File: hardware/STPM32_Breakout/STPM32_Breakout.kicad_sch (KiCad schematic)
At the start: 32 parts, among them J1 BREADBOARD I/O, SW1 RESET, U1 STPM32, Y1 16MHz

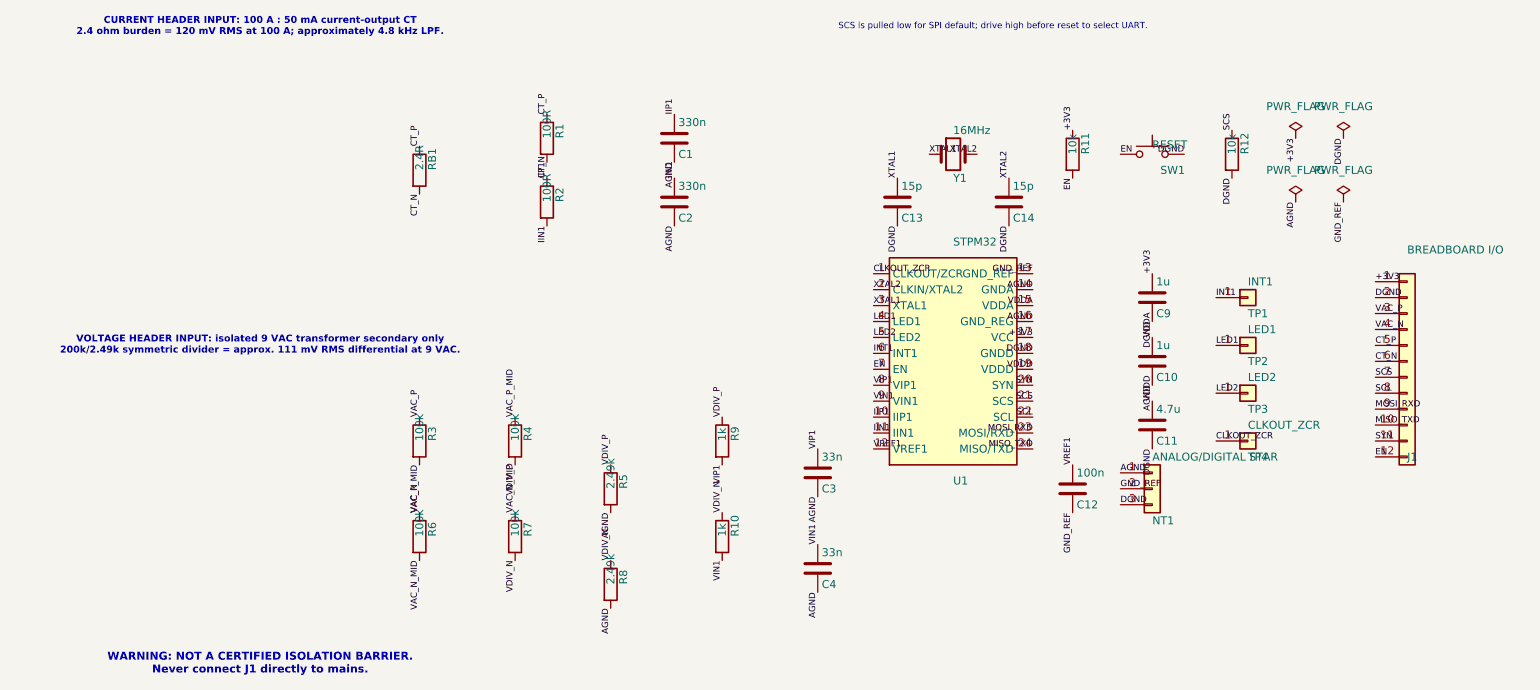
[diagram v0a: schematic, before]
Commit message: Add Elecrow BOM for STPM32
Co-authored-by: Copilot <223556219+Copilot@users.noreply.github.com>
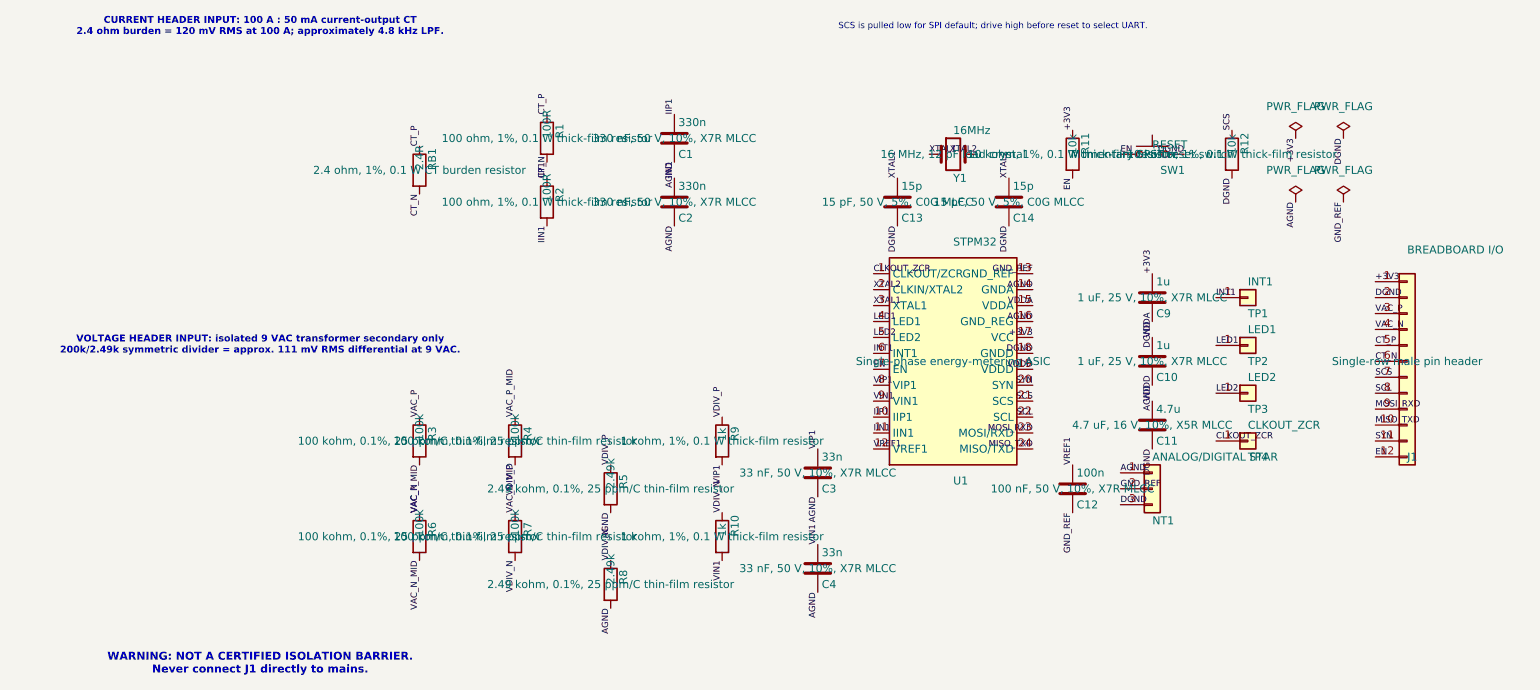
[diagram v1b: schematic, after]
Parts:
- C1, C2: Assembly (none) -> SMT; LCSC (none) -> C282682; MPN (none) -> TCC0603X7R334K500CT; Manufacturer (none) -> CCTC; Package (none) -> 0603 (1608 Metric); Purchase URL (none) -> https://www.lcsc.com/product-detail/C282682.html
- C10, C9: Assembly (none) -> SMT; LCSC (none) -> C116352; MPN (none) -> CL21B105KAFNNNE; Manufacturer (none) -> Samsung Electro-Mechanics; Package (none) -> 0805 (2012 Metric); Purchase URL (none) -> https://www.lcsc.com/product-detail/C116352.html
- C11: Assembly (none) -> SMT; LCSC (none) -> C16194928; MPN (none) -> CL21A475KOFNNNG; Manufacturer (none) -> Samsung Electro-Mechanics; Package (none) -> 0805 (2012 Metric); Purchase URL (none) -> https://www.lcsc.com/product-detail/C16194928.html
- C12: Assembly (none) -> SMT; LCSC (none) -> C1591; MPN (none) -> CL10B104KB8NNNC; Manufacturer (none) -> Samsung Electro-Mechanics; Package (none) -> 0603 (1608 Metric); Purchase URL (none) -> https://www.lcsc.com/product-detail/C1591.html
- C13, C14: Assembly (none) -> SMT; LCSC (none) -> C1644; MPN (none) -> CL10C150JB8NNNC; Manufacturer (none) -> Samsung Electro-Mechanics; Package (none) -> 0603 (1608 Metric); Purchase URL (none) -> https://www.lcsc.com/product-detail/C1644.html
- C3, C4: Assembly (none) -> SMT; LCSC (none) -> C21117; MPN (none) -> CL10B333KB8NNNC; Manufacturer (none) -> Samsung Electro-Mechanics; Package (none) -> 0603 (1608 Metric); Purchase URL (none) -> https://www.lcsc.com/product-detail/C21117.html
- J1: Assembly (none) -> THT; LCSC (none) -> C2840012; MPN (none) -> PZ254V-11-12P; Manufacturer (none) -> XFCN; Notes (none) -> Quote THT assembly separately and confirm pin protrusion su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; Package (none) -> 1x12, 2.54 mm pitch, vertical THT; Purchase URL (none) -> https://www.lcsc.com/product-detail/C2840012.html
- NT1, TP1, TP2, TP3, TP4: now left out of the parts list
- R1, R2: Assembly (none) -> SMT; LCSC (none) -> C105588; MPN (none) -> RC0603FR-07100RL; Manufacturer (none) -> YAGEO; Package (none) -> 0603 (1608 Metric); Purchase URL (none) -> https://www.lcsc.com/product-detail/C105588.html
- R10, R9: Assembly (none) -> SMT; LCSC (none) -> C22548; MPN (none) -> RC0603FR-071KL; Manufacturer (none) -> YAGEO; Package (none) -> 0603 (1608 Metric); Purchase URL (none) -> https://www.lcsc.com/product-detail/C22548.html
- R11, R12: Assembly (none) -> SMT; LCSC (none) -> C98220; MPN (none) -> RC0603FR-0710KL; Manufacturer (none) -> YAGEO; Package (none) -> 0603 (1608 Metric); Purchase URL (none) -> https://www.lcsc.com/product-detail/C98220.html
- R3, R4, R6, R7: Assembly (none) -> SMT; LCSC (none) -> C122538; MPN (none) -> RT0603BRD07100KL; Manufacturer (none) -> YAGEO; Notes (none) -> Use one lot for all four voltage-divider resistors.; Package (none) -> 0603 (1608 Metric); Purchase URL (none) -> https://www.lcsc.com/product-detail/C122538.html
- R5, R8: Assembly (none) -> SMT; LCSC (none) -> C861299; MPN (none) -> RT0603BRD072K49L; Manufacturer (none) -> YAGEO; Notes (none) -> Use one lot for the matched voltage-divider low sides.; Package (none) -> 0603 (1608 Metric); Purchase URL (none) -> https://www.lcsc.com/product-detail/C861299.html
- RB1: Assembly (none) -> SMT; LCSC (none) -> C137746; MPN (none) -> RC0603FR-072R4L; Manufacturer (none) -> YAGEO; Notes (none) -> About 6 mW at 50 mA RMS. The 200 ppm/C TCR is suitable for 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; Package (none) -> 0603 (1608 Metric); Purchase URL (none) -> https://www.lcsc.com/product-detail/C137746.html
- SW1: Assembly (none) -> SMT; LCSC (none) -> C221930; MPN (none) -> RS-282G05A3-SMRT; Manufacturer (none) -> C&K; Package (none) -> C&K RS-282G05A3 SMD; Purchase URL (none) -> https://www.lcsc.com/product-detail/C221930.html
- U1: Assembly (none) -> SMT; LCSC (none) -> C128380; MPN (none) -> STPM32TR; Manufacturer (none) -> STMicroelectronics; Notes (none) -> Inspect exposed-pad paste and voiding during DFM review.; Package (none) -> VQFN-24-EP, 4 x 4 mm, 0.5 mm pitch; Purchase URL (none) -> https://www.lcsc.com/product-detail/C128380.html
- Y1: Assembly (none) -> SMT; LCSC (none) -> C12668; MPN (none) -> X322516MOB4SI; Manufacturer (none) -> YXC; Notes (none) -> 12 pF load is consistent with two 15 pF capacitors plus est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; Package (none) -> SMD3225-4P; Purchase URL (none) -> https://www.lcsc.com/product-detail/C12668.html
